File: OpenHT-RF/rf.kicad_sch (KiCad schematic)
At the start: 42 parts, among them J501 EMPCB.CSMAFSTJ.A, J502 Conn_01x02, J503 Conn_01x02, J504 MS300-10F, J505 MS300-10C, SW501 RFSW8008, U501 AT86RF215, X501 ECS-TXO-20CSMV

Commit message: Added MPN for generic components
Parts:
- C501, C517, C518, C519, C520, C521: MPN (none) -> Generic C/0.1uF/0402/X7R/16V
- C502, C503: MPN (none) -> Generic C/1.8pF/0402/C0G/10V
- C504, C523: MPN (none) -> Generic C/1nF/0402/X7R/10V
- C505: MPN (none) -> Generic C/1nF/0402/C0G/10V
- C506: MPN (none) -> Generic C/10pF/0402/C0G/10V
- C507: MPN (none) -> Generic C/0.8pF/0402/C0G/10V
- C508, C514, C515: MPN (none) -> Generic C/1uF/0402/X5R/10V
- C509, C510, C513: MPN (none) -> Generic C/100pF/0402/C0G/10V
- C511: MPN (none) -> Generic C/220pF/0402/C0G/10V
- C512: MPN (none) -> Generic C/82pF/0402/C0G/10V
- C516: MPN (none) -> Generic C/2.2pF/0402/C0G/10V
- C522: MPN (none) -> Generic C/10uF/0805/X5R/10V
- R3: MPN (none) -> Generic R/100kR/0402/1%
- R402: MPN (none) -> Generic R/100R/0402/1%
- R501: MPN (none) -> Generic R/10kR/0402/1%
- R503: MPN (none) -> Generic R/220R/0402/1%
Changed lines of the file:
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@@
+      (effects (font (size 1.27 1.27)) hide)
+    )
+    (property "MPN" "Generic C/1nF/0402/X7R/10V" (at 199.39 153.67 0)
       (effects (font (size 1.27 1.27)) hide)
     )
@@
       (effects (font (size 1.27 1.27)) hide)
     )
+    (property "MPN" "Generic C/0.1uF/0402/X7R/16V" (at 46.99 72.39 0)
+      (effects (font (size 1.27 1.27)) hide)
+    )
     (pin "1")
     (pin "2")
@@
       (effects (font (size 1.27 1.27)) hide)
     )
+    (property "MPN" "Generic R/10kR/0402/1%" (at 90.17 76.2 0)
+      (effects (font (size 1.27 1.27)) hide)
+    )
     (pin "1")
     (pin "2")
@@
     (property "Dielectric" "C0G" (at 58.42 143.51 90)
       (effects (font (size 1.27 1.27)))
+    )
+    (property "MPN" "Generic C/1.8pF/0402/C0G/10V" (at 58.42 139.7 0)
+      (effects (font (size 1.27 1.27)) hide)
     )
     (pin "1")
@@
       (effects (font (size 1.27 1.27)) (justify left))
     )
+    (property "MPN" "Generic C/220pF/0402/C0G/10V" (at 187.96 128.27 0)
+      (effects (font (size 1.27 1.27)) hide)
+    )
     (pin "1")
     (pin "2")
@@
       (effects (font (size 1.27 1.27)) (justify left))
     )
+    (property "MPN" "Generic C/82pF/0402/C0G/10V" (at 201.93 128.27 0)
+      (effects (font (size 1.27 1.27)) hide)
+    )
     (pin "1")
     (pin "2")
@@
     (property "Dielectric" "C0G" (at 58.42 128.27 90)
       (effects (font (size 1.27 1.27)))
+    )
+    (property "MPN" "Generic C/1.8pF/0402/C0G/10V" (at 58.42 124.46 0)
+      (effects (font (size 1.27 1.27)) hide)
     )
     (pin "1")
@@
       (effects (font (size 1.27 1.27)) hide)
     )
+    (property "MPN" "Generic C/1uF/0402/X5R/10V" (at 114.3 76.2 0)
+      (effects (font (size 1.27 1.27)) hide)
+    )
     (pin "1")
     (pin "2")
@@
     (property "Dielectric" "C0G" (at 96.52 80.645 0)
       (effects (font (size 1.27 1.27)))
+    )
+    (property "MPN" "Generic C/10pF/0402/C0G/10V" (at 101.6 76.2 0)
+      (effects (font (size 1.27 1.27)) hide)
     )
     (pin "1")
@@
       (effects (font (size 1.27 1.27)) hide)
     )
+    (property "MPN" "Generic C/1uF/0402/X5R/10V" (at 195.58 90.17 0)
+      (effects (font (size 1.27 1.27)) hide)
+    )
     (pin "1")
     (pin "2")
@@
     (property "Dielectric" "C0G" (at 97.79 175.26 0)
       (effects (font (size 1.27 1.27)) (justify left))
+    )
+    (property "MPN" "Generic C/1nF/0402/C0G/10V" (at 93.98 170.18 0)
+      (effects (font (size 1.27 1.27)) hide)
     )
     (pin "1")
@@
       (effects (font (size 1.27 1.27)) hide)
     )
+    (property "MPN" "Generic C/0.1uF/0402/X7R/16V" (at 81.28 99.06 0)
+      (effects (font (size 1.27 1.27)) hide)
+    )
     (pin "1")
     (pin "2")
@@
       (effects (font (size 1.27 1.27)) hide)
     )
+    (property "MPN" "Generic C/0.1uF/0402/X7R/16V" (at 87.63 99.06 0)
+      (effects (font (size 1.27 1.27)) hide)
+    )
     (pin "1")
     (pin "2")
@@
       (effects (font (size 1.27 1.27)))
     )
+    (property "MPN" "Generic C/100pF/0402/C0G/10V" (at 153.67 162.56 0)
+      (effects (font (size 1.27 1.27)) hide)
+    )
     (pin "1")
     (pin "2")
@@
     )
     (property "Datasheet" "~" (at 83.82 67.31 0)
+      (effects (font (size 1.27 1.27)) hide)
+    )
+    (property "MPN" "Generic C/1nF/0402/X7R/10V" (at 83.82 67.31 0)
       (effects (font (size 1.27 1.27)) hide)
     )
@@
       (effects (font (size 1.27 1.27)) hide)
     )
+    (property "MPN" "Generic C/10uF/0805/X5R/10V" (at 50.8 31.75 0)
+      (effects (font (size 1.27 1.27)) hide)
+    )
     (pin "1")
     (pin "2")
@@
     )
     (property "Tolerance" "1%" (at 120.65 63.5 0)
+      (effects (font (size 1.27 1.27)) hide)
+    )
+    (property "MPN" "Generic R/100kR/0402/1%" (at 120.65 63.5 0)
       (effects (font (size 1.27 1.27)) hide)
     )
@@
       (effects (font (size 1.27 1.27)))
     )
+    (property "MPN" "Generic C/100pF/0402/C0G/10V" (at 153.67 129.54 0)
+      (effects (font (size 1.27 1.27)) hide)
+    )
     (pin "1")
     (pin "2")
@@
       (effects (font (size 1.27 1.27)) (justify right))
     )
+    (property "MPN" "Generic C/2.2pF/0402/C0G/10V" (at 91.44 55.88 0)
+      (effects (font (size 1.27 1.27)) hide)
+    )
     (pin "1")
     (pin "2")
@@
     )
     (property "Tolerance" "1%" (at 147.32 34.29 90)
+      (effects (font (size 1.27 1.27)) hide)
+    )
+    (property "MPN" "Generic R/100R/0402/1%" (at 147.32 34.29 0)
       (effects (font (size 1.27 1.27)) hide)
     )
@@
     )
     (property "Datasheet" "~" (at 199.39 55.88 0)
+      (effects (font (size 1.27 1.27)) hide)
+    )
+    (property "MPN" "Generic C/1uF/0402/X5R/10V" (at 199.39 55.88 0)
       (effects (font (size 1.27 1.27)) hide)
     )
@@
       (effects (font (size 1.27 1.27)) hide)
     )
+    (property "MPN" "Generic C/0.1uF/0402/X7R/16V" (at 48.26 99.06 0)
+      (effects (font (size 1.27 1.27)) hide)
+    )
     (pin "1")
     (pin "2")
@@
     )
     (property "Datasheet" "~" (at 59.69 99.06 0)
+      (effects (font (size 1.27 1.27)) hide)
+    )
+    (property "MPN" "Generic C/0.1uF/0402/X7R/16V" (at 59.69 99.06 0)
       (effects (font (size 1.27 1.27)) hide)
     )
@@
       (effects (font (size 1.27 1.27)))
     )
+    (property "MPN" "Generic C/0.8pF/0402/C0G/10V" (at 107.95 162.56 0)
+      (effects (font (size 1.27 1.27)) hide)
+    )
     (pin "1")
     (pin "2")
@@
       (effects (font (size 1.27 1.27)) hide)
     )
+    (property "MPN" "Generic R/220R/0402/1%" (at 99.06 50.8 0)
+      (effects (font (size 1.27 1.27)) hide)
+    )
     (pin "1")
     (pin "2")
@@
       (effects (font (size 1.27 1.27)) hide)
     )
+    (property "MPN" "Generic C/0.1uF/0402/X7R/16V" (at 36.83 99.06 0)
+      (effects (font (size 1.27 1.27)) hide)
+    )
     (pin "1")
     (pin "2")
@@
       (effects (font (size 1.27 1.27)))
     )
-    (pin "1")
+    (property "MPN" "Generic C/100pF/0402/C0G/10V" (at 213.36 146.05 0)
+      (effects (font (size 1.27 1.27)) hide)
+    )
+    (pin "1")

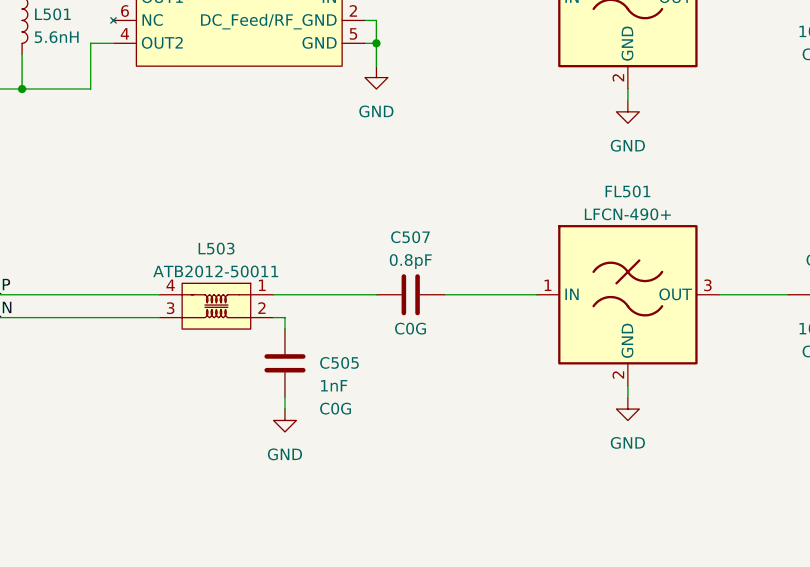
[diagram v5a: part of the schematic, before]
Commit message: Removed C507
Addresses #4
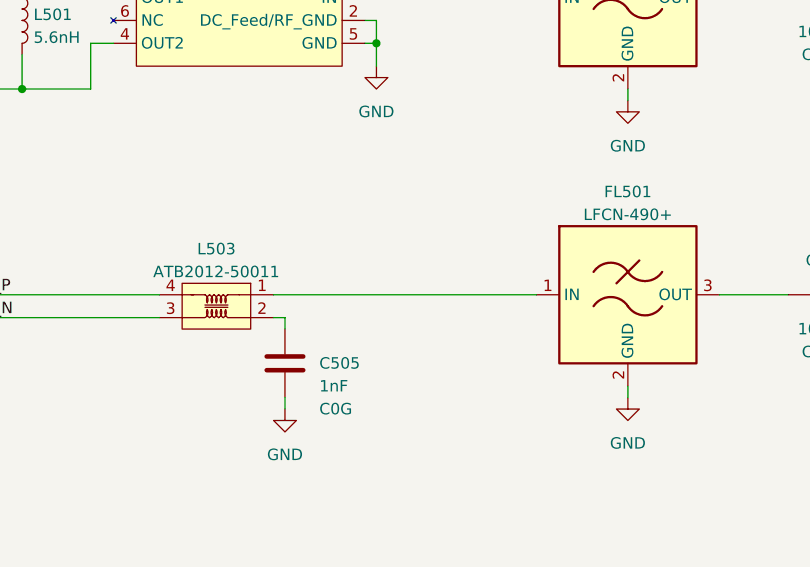
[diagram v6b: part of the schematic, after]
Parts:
- removed C507: 0.8pF, Capacitor_SMD:C_0402_1005Metric, symbol Device:C
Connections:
- net at L503.1: now also FL501.1 (IN)
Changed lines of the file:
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@@
     (stroke (width 0) (type default))
   )
-  (wire (pts (xy 92.71 162.56) (xy 104.14 162.56))
+  (wire (pts (xy 92.71 162.56) (xy 121.92 162.56))
     (stroke (width 0) (type default))
   )
@@
   )
   (wire (pts (xy 187.96 123.19) (xy 187.96 124.46))
-    (stroke (width 0) (type default))
-  )
-  (wire (pts (xy 111.76 162.56) (xy 121.92 162.56))
     (stroke (width 0) (type default))
   )
@@
     (effects (font (size 1.27 1.27)) (justify left bottom))
     (property "Netclass" "50Ohm" (at 144.2085 127 0)
-      (effects (font (size 1.27 1.27) italic) (justify left))
-    )
-  )
-  (netclass_flag "" (length 2.54) (shape round) (at 114.3 162.56 0) (fields_autoplaced)
-    (effects (font (size 1.27 1.27)) (justify left bottom))
-    (property "Netclass" "50Ohm" (at 114.9985 160.02 0)
       (effects (font (size 1.27 1.27) italic) (justify left))
     )
@@
         )
       )
-    )
-  )
-  (symbol (lib_id "Device:C") (at 107.95 162.56 90) (unit 1)
-    (in_bom yes) (on_board yes) (dnp no)
-    (property "Reference" "C507" (at 107.95 156.21 90)
-      (effects (font (size 1.27 1.27)))
-    )
-    (property "Value" "0.8pF" (at 107.95 158.75 90)
-      (effects (font (size 1.27 1.27)))
-    )
-    (property "Footprint" "Capacitor_SMD:C_0402_1005Metric" (at 111.76 161.5948 0)
-      (effects (font (size 1.27 1.27)) hide)
-    )
-    (property "Datasheet" "~" (at 107.95 162.56 0)
-      (effects (font (size 1.27 1.27)) hide)
-    )
-    (property "Dielectric" "C0G" (at 107.95 166.37 90)
-      (effects (font (size 1.27 1.27)))
-    )
-    (property "MPN" "Generic C/0.8pF/0402/C0G/10V" (at 107.95 162.56 0)
-      (effects (font (size 1.27 1.27)) hide)
-    )
-    (pin "1")
-    (pin "2")
-    (instances
-      (project "OpenHT-RF"
-        (path "/3c300b59-23ec-47f8-bb91-29ca34130bcf/e3bba2b3-d2df-4b56-8e13-359b6c4f2426"
-          (reference "C507") (unit 1)
-        )
-      )
